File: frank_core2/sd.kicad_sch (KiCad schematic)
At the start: 2 parts, among them J7 104031-0811

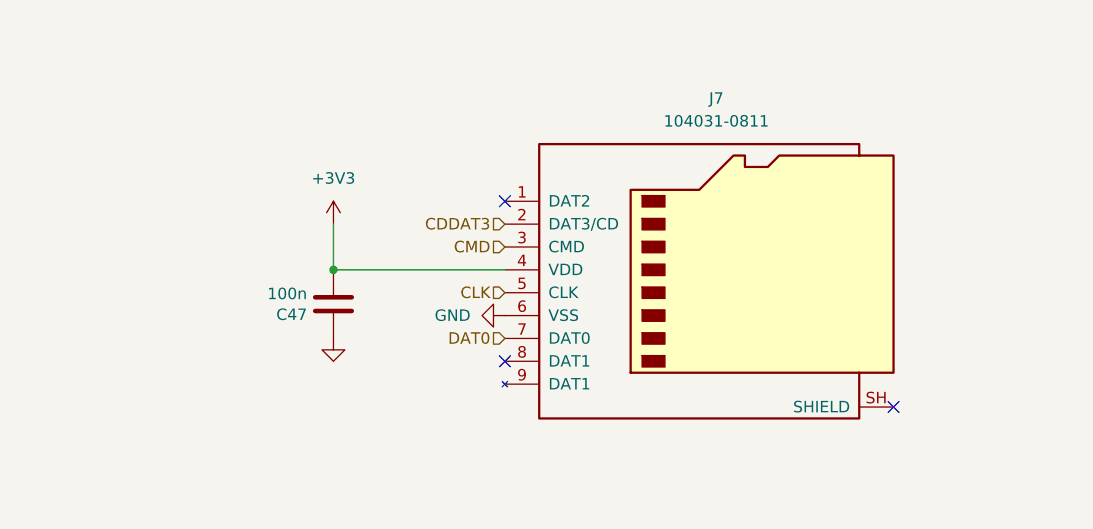
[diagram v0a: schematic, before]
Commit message: Boards WIP
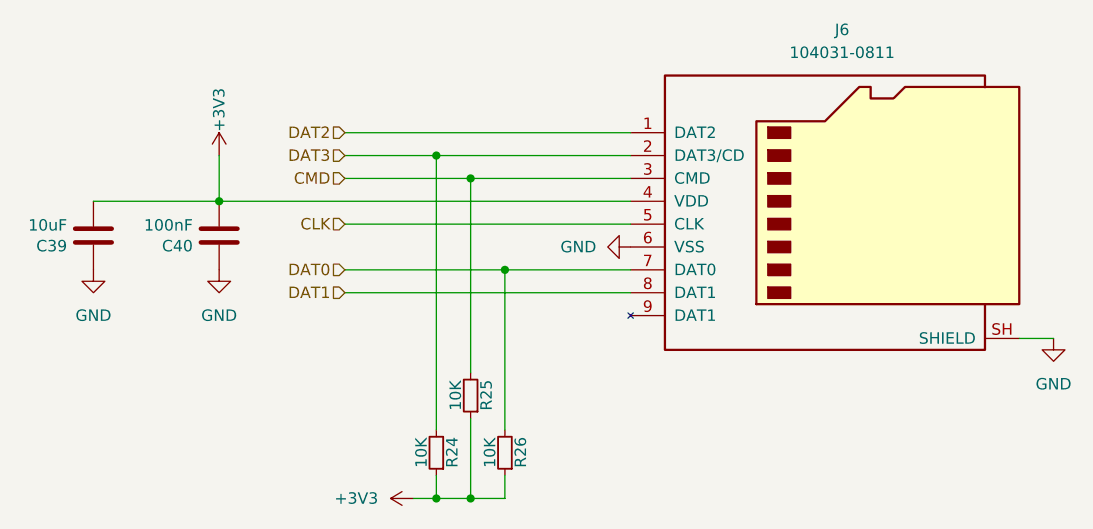
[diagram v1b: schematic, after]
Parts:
- added C39: 10uF, FRANK:C_0603_1608Metric, symbol FRANK:C
- added R24, R25, R26: 10K, FRANK:R_0603_1608Metric, symbol FRANK:R_Small
- C40: renamed from C47; value 100n -> 100nF; LCSC (none) -> C14663
- J6: renamed from J7; LCSC (none) -> C585350
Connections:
- net +3V3: now also C39.2, R24.1, R25.1, R26.1
- net CMD: now also R25.2
- net DAT0: now also R26.2
- net GND: now also J6.SH (SHIELD), C39.1
- net DAT2: now reaches J6.1 (DAT2)
- net DAT1: now reaches J6.8 (DAT1)
- net CDDAT3 renamed DAT3
- net DAT3: now also R24.2
- no-connect marks 3 -> 0
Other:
- moved on the sheet: C40, J6
